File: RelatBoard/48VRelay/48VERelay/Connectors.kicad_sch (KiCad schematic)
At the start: 5 parts, among them J2 RJ45_Hanrun_HR911105A_Horizon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, J3 B4B-PH-SM4-TB, J5 TC2030

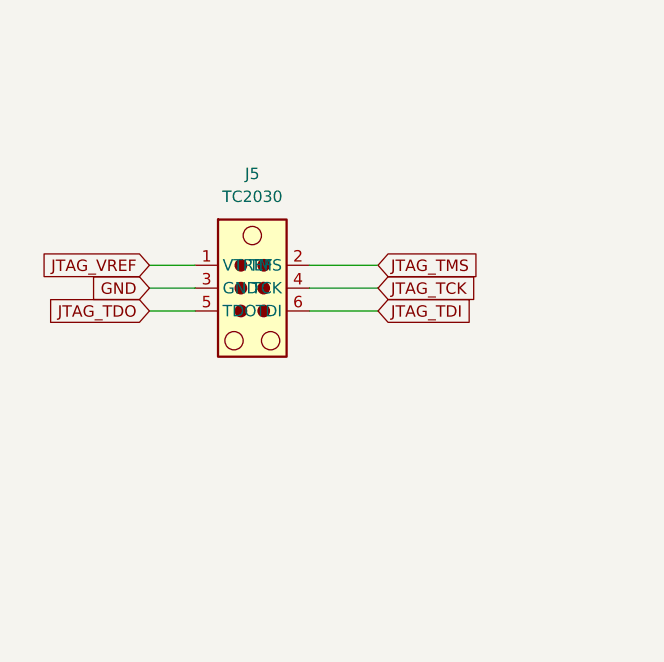
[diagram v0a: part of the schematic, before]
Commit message: Final design
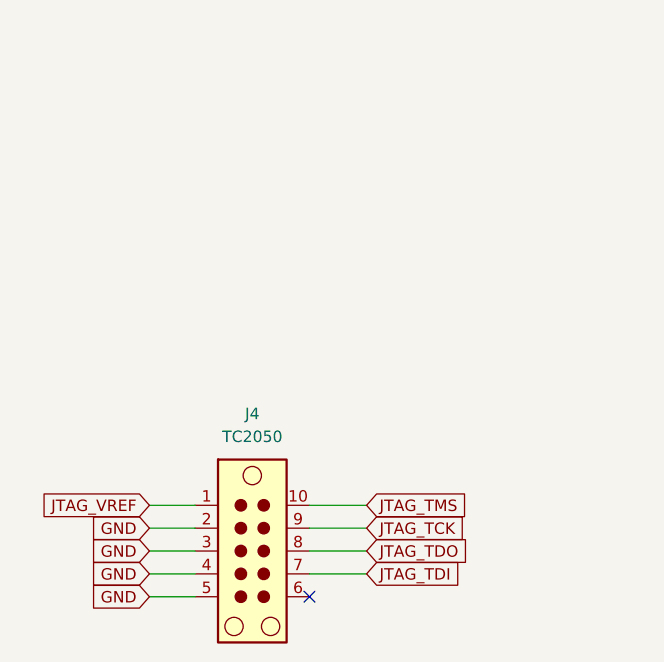
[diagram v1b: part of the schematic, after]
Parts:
- removed J5: TC2030, Connector:Tag-Connect_TC2030-IDC-NL_2x03_P1.27mm_Vertical, symbol Connector:TC2030
- added J4: TC2050, Connector:Tag-Connect_TC2050-IDC-NL_2x05_P1.27mm_Vertical, symbol Connector:TC2050
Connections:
- net GND: now also J4.2, J4.3, J4.4, J4.5
- net JTAG_TCK: now also J4.9
- net JTAG_TDI: now also J4.7
- net JTAG_TDO: now also J4.8
- net JTAG_TMS: now also J4.10
- net JTAG_VREF: now also J4.1
- no-connect marks 0 -> 1
